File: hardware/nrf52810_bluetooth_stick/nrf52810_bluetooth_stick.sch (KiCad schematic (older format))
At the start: 32 parts

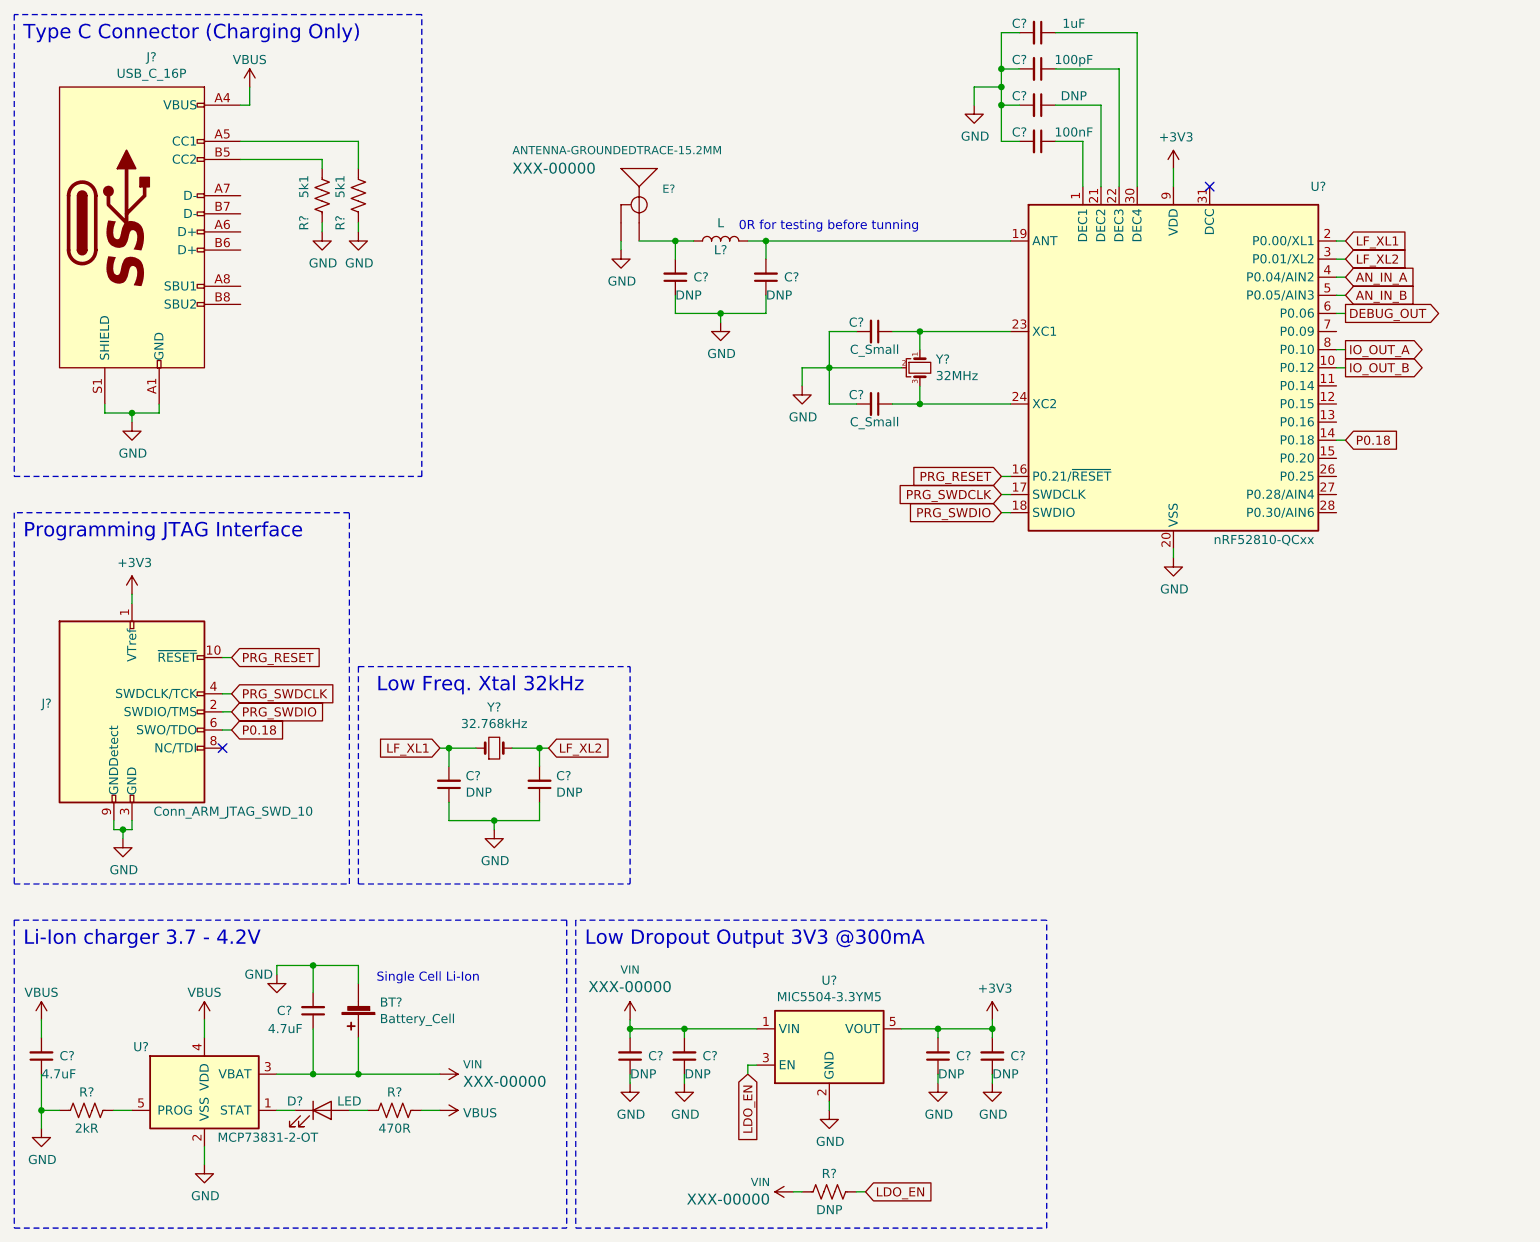
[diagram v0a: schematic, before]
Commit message: Template update...
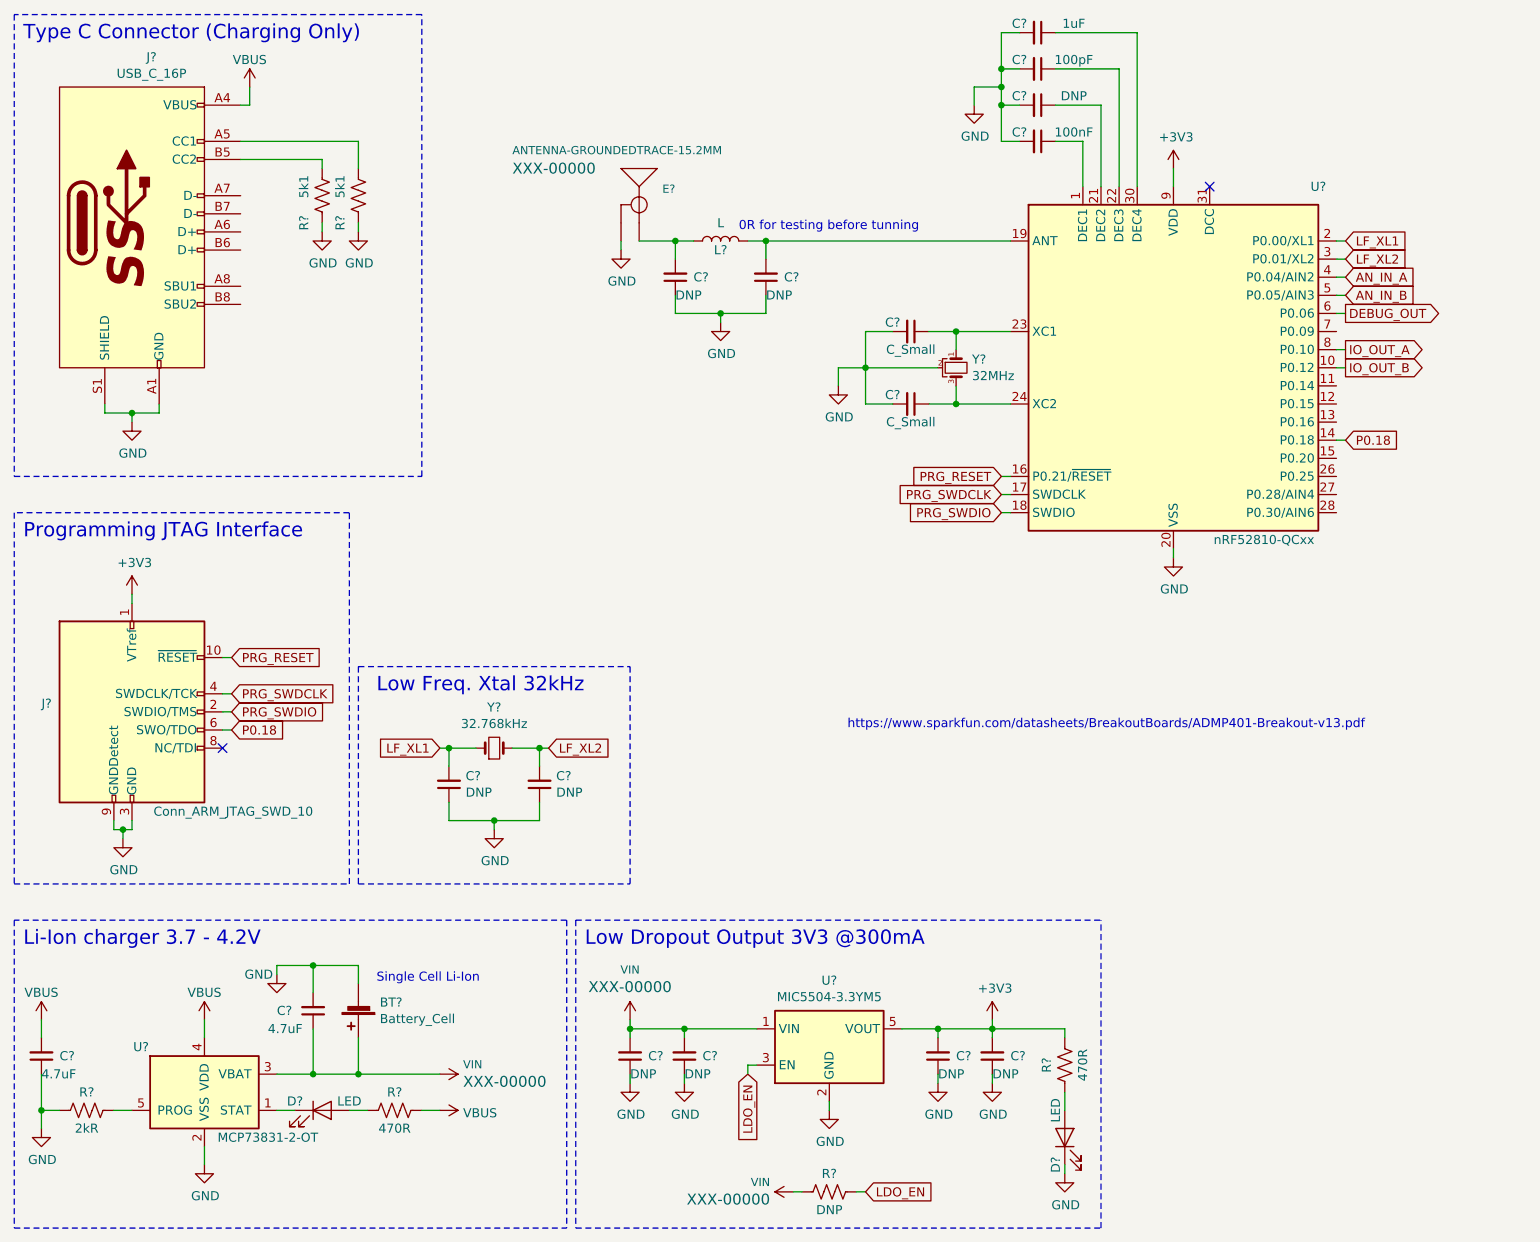
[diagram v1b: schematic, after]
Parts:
- added D?: LED, symbol Device:LED
- added R?: 470R, symbol Device:R_US
- J?: footprint (none) -> Connector_PinHeader_1.27mm:PinHeader_2x05_P1.27mm_Vertical_SMD
- J?: footprint (none) -> Connector_USB:USB_C_Receptacle_Palconn_UTC16-G
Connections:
- net +3V3: now also R?.2
- net GND: now also D?.1 (K)
- new net: D?.2 (A), R?.1
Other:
- note added: "https://www.sparkfun.com/datasheets/BreakoutBoards/ADMP401-Breakout-v13.pdf"
- moved on the sheet: C?, Y?
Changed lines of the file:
@@
 L Device:Crystal_GND2_Small Y?
 U 1 1 5EA575AD
-P 5850 2900
-F 0 "Y?" V 5804 2988 50  0000 L CNN
-F 1 "32MHz" V 5895 2988 50  0000 L CNN
-F 2 "" H 5850 2900 50  0001 C CNN
-F 3 "~" H 5850 2900 50  0001 C CNN
-	1    5850 2900
+P 6050 2900
+F 0 "Y?" V 6004 2988 50  0000 L CNN
+F 1 "32MHz" V 6095 2988 50  0000 L CNN
+F 2 "" H 6050 2900 50  0001 C CNN
+F 3 "~" H 6050 2900 50  0001 C CNN
+	1    6050 2900
 	0    1    1    0
 $EndComp
 Wire Wire Line
-	5850 2800 5850 2700
-Wire Wire Line
-	5850 2700 6350 2700
-Wire Wire Line
-	5850 3000 5850 3100
-Wire Wire Line
-	5850 3100 6350 3100
+	6050 2800 6050 2700
+Wire Wire Line
+	6050 3000 6050 3100
 $Comp
 L Device:C_Small C?
 U 1 1 5EA5940D
-P 5600 2700
-F 0 "C?" V 5550 2600 50  0000 C CNN
-F 1 "C_Small" V 5700 2700 50  0000 C CNN
-F 2 "" H 5600 2700 50  0001 C CNN
-F 3 "~" H 5600 2700 50  0001 C CNN
-	1    5600 2700
+P 5800 2700
+F 0 "C?" V 5750 2600 50  0000 C CNN
+F 1 "C_Small" V 5900 2700 50  0000 C CNN
+F 2 "" H 5800 2700 50  0001 C CNN
+F 3 "~" H 5800 2700 50  0001 C CNN
+	1    5800 2700
 	0    1    1    0
 $EndComp
@@
 L Device:C_Small C?
 U 1 1 5EA5A037
-P 5600 3100
-F 0 "C?" V 5550 3000 50  0000 C CNN
-F 1 "C_Small" V 5700 3100 50  0000 C CNN
-F 2 "" H 5600 3100 50  0001 C CNN
-F 3 "~" H 5600 3100 50  0001 C CNN
-	1    5600 3100
+P 5800 3100
+F 0 "C?" V 5750 3000 50  0000 C CNN
+F 1 "C_Small" V 5900 3100 50  0000 C CNN
+F 2 "" H 5800 3100 50  0001 C CNN
+F 3 "~" H 5800 3100 50  0001 C CNN
+	1    5800 3100
 	0    1    1    0
 $EndComp
 Wire Wire Line
-	5700 2700 5850 2700
-Connection ~ 5850 2700
-Wire Wire Line
-	5700 3100 5850 3100
-Connection ~ 5850 3100
-Wire Wire Line
-	5500 2700 5350 2700
-Wire Wire Line
-	5350 2700 5350 2900
-Wire Wire Line
-	5350 3100 5500 3100
-Wire Wire Line
-	5750 2900 5350 2900
-Connection ~ 5350 2900
-Wire Wire Line
-	5350 2900 5350 3100
+	5900 2700 6050 2700
+Wire Wire Line
+	5900 3100 6050 3100
+Wire Wire Line
+	5700 2700 5550 2700
+Wire Wire Line
+	5550 2700 5550 2900
+Wire Wire Line
+	5550 3100 5700 3100
+Wire Wire Line
+	5950 2900 5550 2900
+Connection ~ 5550 2900
+Wire Wire Line
+	5550 2900 5550 3100
 $Comp
 L power:GND #PWR?
 U 1 1 5EA5AA9B
-P 5200 3000
-F 0 "#PWR?" H 5200 2750 50  0001 C CNN
-F 1 "GND" H 5205 2827 50  0000 C CNN
-F 2 "" H 5200 3000 50  0001 C CNN
-F 3 "" H 5200 3000 50  0001 C CNN
-	1    5200 3000
-	1    0    0    -1
-$EndComp
-Wire Wire Line
-	5350 2900 5200 2900
-Wire Wire Line
-	5200 2900 5200 3000
+P 5400 3000
+F 0 "#PWR?" H 5400 2750 50  0001 C CNN
+F 1 "GND" H 5405 2827 50  0000 C CNN
+F 2 "" H 5400 3000 50  0001 C CNN
+F 3 "" H 5400 3000 50  0001 C CNN
+	1    5400 3000
+	1    0    0    -1
+$EndComp
+Wire Wire Line
+	5550 2900 5400 2900
+Wire Wire Line
+	5400 2900 5400 3000
 Wire Wire Line
 	6350 3500 6300 3500
@@
 F 0 "J?" H 1057 4846 50  0000 R CNN
 F 1 "Conn_ARM_JTAG_SWD_10" H 2500 4250 50  0000 R CNN
-F 2 "" H 1500 4800 50  0001 C CNN
+F 2 "Connector_PinHeader_1.27mm:PinHeader_2x05_P1.27mm_Vertical_SMD" H 1500 4800 50  0001 C CNN
 F 3 "http://infocenter.arm.com/help/topic/com.arm.doc.ddi0314h/DDI0314H_coresight_components_trm.pdf" V 1150 3550 50  0001 C CNN
 	1    1500 4800
@@
 	3950 5950 3950 7650
 Wire Notes Line
-	3950 7650 6550 7650
-Wire Notes Line
-	6550 7650 6550 5950
-Wire Notes Line
-	6550 5950 3950 5950
-Wire Notes Line
 	850  7650 3900 7650
 Wire Notes Line
@@
 F 0 "J?" H 1608 3715 50  0000 C CNN
 F 1 "USB_C_16P" H 1608 3624 50  0000 C CNN
-F 2 "" H 1650 2450 50  0001 C CNN
+F 2 "Connector_USB:USB_C_Receptacle_Palconn_UTC16-G" H 1650 2450 50  0001 C CNN
 F 3 "https://www.usb.org/sites/default/files/documents/usb_type-c.zip" H 1650 2450 50  0001 C CNN
 	1    1500 2450
@@
 Text GLabel 8200 2900 2    50   Output ~ 0
 IO_OUT_B
+$Comp
+L Device:LED D?
+U 1 1 5EC237B6
+P 6650 7150
+F 0 "D?" H 6500 7200 50  0000 C CNN
+F 1 "LED" H 6800 7200 50  0000 C CNN
+F 2 "" H 6650 7150 50  0001 C CNN
+F 3 "~" H 6650 7150 50  0001 C CNN
+	1    6650 7150
+	0    -1   -1   0
+$EndComp
+$Comp
+L Device:R_US R?
+U 1 1 5EC237BC
+P 6650 6750
+F 0 "R?" V 6750 6750 50  0000 C CNN
+F 1 "470R" V 6550 6750 50  0000 C CNN
+F 2 "" V 6690 6740 50  0001 C CNN
+F 3 "~" H 6650 6750 50  0001 C CNN
+	1    6650 6750
+	-1   0    0    1
+$EndComp
+Wire Wire Line
+	6650 7000 6650 6900
+Wire Wire Line
+	6250 6550 6650 6550
+Wire Wire Line
+	6650 6550 6650 6600
+$Comp
+L power:GND #PWR?
+U 1 1 5EC353F6
+P 6650 7350
+F 0 "#PWR?" H 6650 7100 50  0001 C CNN
+F 1 "GND" H 6655 7177 50  0000 C CNN
+F 2 "" H 6650 7350 50  0001 C CNN
+F 3 "" H 6650 7350 50  0001 C CNN
+	1    6650 7350
+	1    0    0    -1
+$EndComp
+Wire Wire Line
+	6650 7350 6650 7300
+Wire Notes Line
+	6850 7650 6850 5950
+Wire Notes Line
+	3950 7650 6850 7650
+Wire Notes Line
+	3950 5950 6850 5950
+Wire Wire Line
+	6350 2700 6050 2700
+Connection ~ 6050 2700
+Wire Wire Line
+	6350 3100 6050 3100
+Connection ~ 6050 3100
+Text Notes 5450 4900 0    50   ~ 0
+https://www.sparkfun.com/datasheets/BreakoutBoards/ADMP401-Breakout-v13.pdf
 $EndSCHEMATC
